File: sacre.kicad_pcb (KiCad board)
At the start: 2 copper layers, 91.4 x 88.4 mm, 72 parts, among them IC1 ST25DV64KC-IE6S3, J1 USB_B_Micro, J2 Conn_01x24, J3 Con_BATT, M1 Vibration_Motor, Q1 DMP1045U_GSD, Q2 UMH3N, Q3 S8050, Q4 SI1308EDL, SW1 SW, SW2 SW, SW3 SW, SW4 SW, U1 TP4054, U2 ADP2108AUJ-3.3, U3 CP2104, U4 LIS3DH, U5 ESP32-PICO-D4, Y1 RV-8803-C7-TA-QC

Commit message: Clean KiCad project files
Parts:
- S1: footprint SamacSys_Parts:MSK12C02 -> MSK12C02:MSK12C02
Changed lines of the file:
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@@
     (pad "3" smd rect locked (at -2.625 -0.85) (size 1 1.55) (layers "F.Cu" "F.Paste" "F.Mask"))
     (pad "4" smd rect locked (at -2.625 0.85) (size 1 1.55) (layers "F.Cu" "F.Paste" "F.Mask"))
-    (model "EVQ-PUA02K.stp"
-      (offset (xyz 0 0 0))
-      (scale (xyz 1 1 1))
-      (rotate (xyz 0 0 0))
-    )
-    (model "${KICAD6_3DMODEL_DIR}/EVQ-PUA02K.3dshapes/EVQ-PUA02K.stp"
+    (model "${KIPRJMOD}/EVQ-PUA02K/EVQ-PUA02K.stp"
       (offset (xyz 0 0 0))
       (scale (xyz 1 1 1))
@@
     (pad "3" smd rect locked (at -2.625 -0.85 180) (size 1 1.55) (layers "F.Cu" "F.Paste" "F.Mask"))
     (pad "4" smd rect locked (at -2.625 0.85 180) (size 1 1.55) (layers "F.Cu" "F.Paste" "F.Mask"))
-    (model "EVQ-PUA02K.stp"
-      (offset (xyz 0 0 0))
-      (scale (xyz 1 1 1))
-      (rotate (xyz 0 0 0))
-    )
-    (model "${KICAD6_3DMODEL_DIR}/EVQ-PUA02K.3dshapes/EVQ-PUA02K.stp"
+    (model "${KIPRJMOD}/EVQ-PUA02K/EVQ-PUA02K.stp"
       (offset (xyz 0 0 0))
       (scale (xyz 1 1 1))
@@
     (pad "3" smd rect locked (at -2.625 -0.85 180) (size 1 1.55) (layers "F.Cu" "F.Paste" "F.Mask"))
     (pad "4" smd rect locked (at -2.625 0.85 180) (size 1 1.55) (layers "F.Cu" "F.Paste" "F.Mask"))
-    (model "EVQ-PUA02K.stp"
-      (offset (xyz 0 0 0))
-      (scale (xyz 1 1 1))
-      (rotate (xyz 0 0 0))
-    )
-    (model "${KICAD6_3DMODEL_DIR}/EVQ-PUA02K.3dshapes/EVQ-PUA02K.stp"
+    (model "${KIPRJMOD}/EVQ-PUA02K/EVQ-PUA02K.stp"
       (offset (xyz 0 0 0))
       (scale (xyz 1 1 1))
@@
     (pad "2" smd rect locked (at 1.425 0 90) (size 1.55 3) (layers "F.Cu" "F.Paste" "F.Mask")
       (net 4 "+3V3") (pintype "passive"))
-    (model "LQH44PN100MP0L.stp"
-      (offset (xyz 0 0 0))
-      (scale (xyz 1 1 1))
-      (rotate (xyz 0 0 0))
-    )
   )
   (footprint "Diode_SMD:D_SOD-123" locked (layer "F.Cu")
@@
     )
   )
-  (footprint "SamacSys_Parts:MSK12C02" locked (layer "F.Cu")
+  (footprint "MSK12C02:MSK12C02" locked (layer "F.Cu")
     (at 53.7 156.5)
     (descr "MSK12C02-1")
@@
     (pad "MP4" smd rect locked (at -3.45 -1.05 90) (size 0.5 0.8) (layers "F.Cu" "F.Paste" "F.Mask")
       (net 56 "Net-(S1-PadMP1)") (pinfunction "MP4") (pintype "passive"))
-    (model "C:\\Users\\Cosmin\\Desktop\\KiCadLib\\SamacSys_Parts.3dshapes\\MSK12C02.stp"
-      (offset (xyz 0 0 0.7))
-      (scale (xyz 1 1 1))
-      (rotate (xyz -90 0 0))
-    )
   )
   (footprint "Inductor_SMD:L_0805_2012Metric_Pad1.15x1.40mm_HandSolder" locked (layer "F.Cu")
@@
     (pad "3" smd rect locked (at -2.625 -0.85) (size 1 1.55) (layers "F.Cu" "F.Paste" "F.Mask"))
     (pad "4" smd rect locked (at -2.625 0.85) (size 1 1.55) (layers "F.Cu" "F.Paste" "F.Mask"))
-    (model "EVQ-PUA02K.stp"
-      (offset (xyz 0 0 0))
-      (scale (xyz 1 1 1))
-      (rotate (xyz 0 0 0))
-    )
-    (model "${KICAD6_3DMODEL_DIR}/EVQ-PUA02K.3dshapes/EVQ-PUA02K.stp"
-      (offset (xyz 0 0 0))
-      (scale (xyz 1 1 1))
+    (model "${KIPRJMOD}/EVQ-PUA02K/EVQ-PUA02K.stp"
+      (offset (xyz 0 0 0))
+      (scale (xyz 1 1 1))

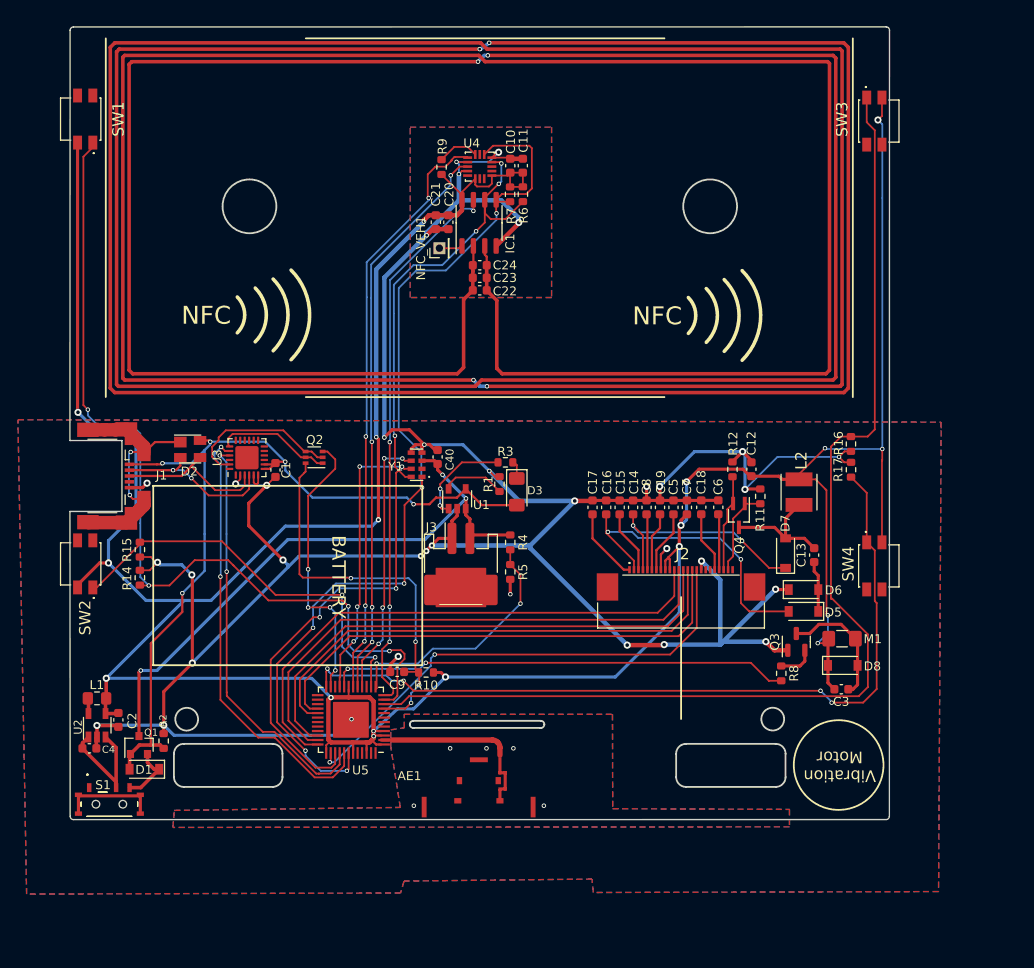
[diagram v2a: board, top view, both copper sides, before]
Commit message: se fini
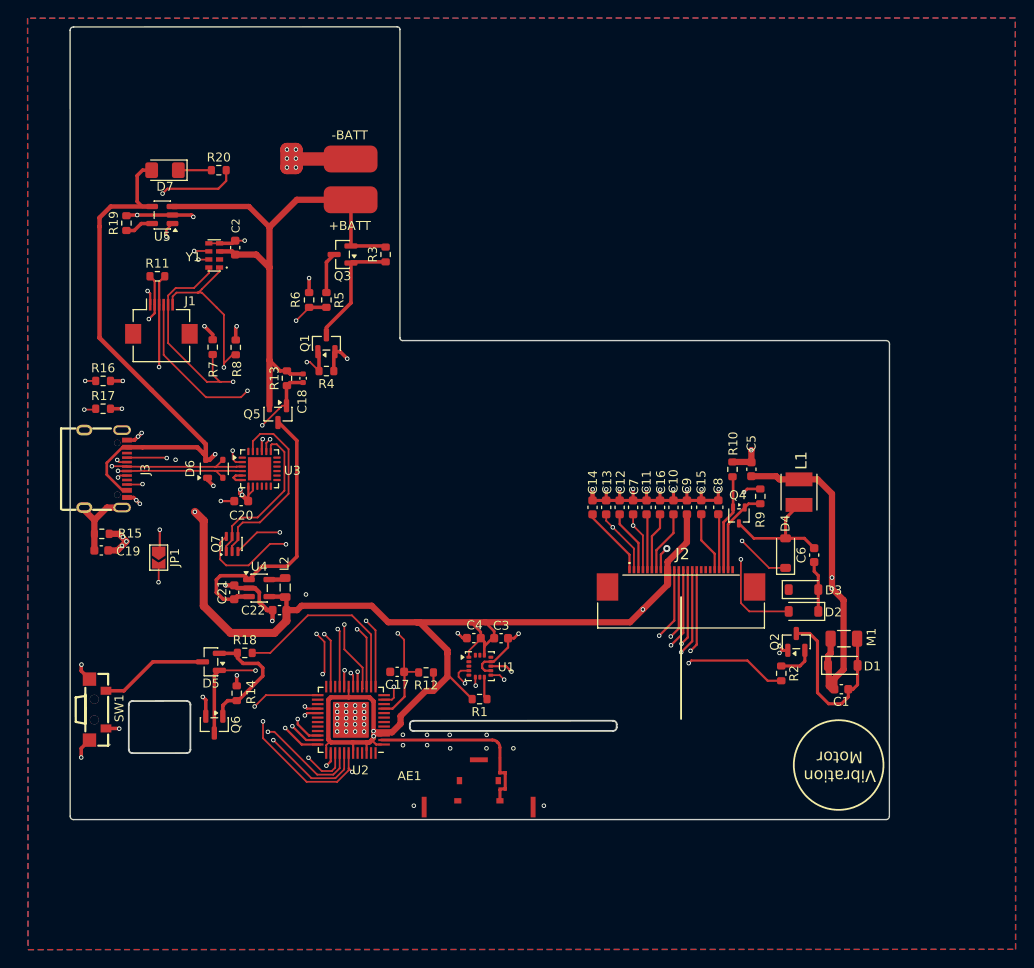
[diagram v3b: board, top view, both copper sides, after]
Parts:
- removed the C1 at (72.2, 119.2)
- removed the C10 at (98.4, 85.3)
- removed the C11 at (99.8, 85.3)
- removed the C2 at (54.7, 147.1)
- removed C23, C24: C_Tune, Capacitor_SMD:C_0603_1608Metric
- removed the D1 at (57.6, 152.6)
- removed the D2 at (62.7, 116.9)
- removed the D3 at (99.1, 121.7)
- removed IC1: ST25DV64KC-IE6S3, Package_SO:SO-8_3.9x4.9mm_P1.27mm
- removed the L1 at (52.3, 144.7)
- removed NFC_VEH1: Conn_01x01_Female, Connector_PinHeader_2.00mm:PinHeader_1x01_P2.00mm_Vertical
- removed the Q2 at (76.5, 117.8)
- removed the R2 at (59.8, 149.4)
- removed the R9 at (90.7, 85.5)
- removed S1: MSK12C02, MSK12C02:MSK12C02
- removed SW2, SW3, SW4: SW, EVQ-PUA02K:EVQPUA02K
- removed the U2 at (52.3, 147.7)
- added C18: 100nF, Capacitor_SMD:C_0402_1005Metric, F.Cu at (75.3, 109.0)
- added C19: 4.7nF, Capacitor_SMD:C_0603_1608Metric, F.Cu at (52.8, 128.2)
- added C3: 0.1uF, Capacitor_SMD:C_0603_1608Metric, F.Cu at (97.4, 138.0)
- added D5: BAT54C, Package_TO_SOT_SMD:SOT-23, F.Cu at (65.0, 140.6)
- added D6: SP0503BAHTG, Package_TO_SOT_SMD:SOT-143, F.Cu at (65.4, 119.1)
- added D7: LED, LED_SMD:LED_1206_3216Metric_Pad1.42x1.75mm_HandSolder, F.Cu at (59.9, 85.8)
- added J5: +BATT, Connector_Wire:SolderWirePad_1x01_SMD_3x6mm, F.Cu at (80.6, 89.1)
- added J6: -BATT, Connector_Wire:SolderWirePad_1x01_SMD_3x6mm, F.Cu at (80.6, 84.5)
- added JP1: Jumper_RES_Touch, Jumper:SolderJumper-2_P1.3mm_Open_TrianglePad1.0x1.5mm, F.Cu at (59.2, 129.0)
- added L2: 1uH, Inductor_SMD:L_0805_2012Metric, F.Cu at (73.3, 132.3)
- added Q3: CJ3415, Package_TO_SOT_SMD:SOT-23, F.Cu at (79.7, 95.2)
- added Q5: CJ3415, Package_TO_SOT_SMD:SOT-23, F.Cu at (72.5, 113.0)
- added Q6: CJ2312, Package_TO_SOT_SMD:SOT-23, F.Cu at (65.4, 147.6)
- added Q7: UMH3N, Package_TO_SOT_SMD:SOT-363_SC-70-6, F.Cu at (67.4, 127.5)
- added R11: 10K, Resistor_SMD:R_0603_1608Metric, F.Cu at (59.0, 97.6)
- added R13: 300k, Resistor_SMD:R_0603_1608Metric, F.Cu at (73.5, 109.0)
- added R18: 1k, Resistor_SMD:R_0603_1608Metric, F.Cu at (68.8, 139.6)
- added R19: 10K, Resistor_SMD:R_0603_1608Metric, F.Cu at (55.6, 91.7)
- added R20: 1K, Resistor_SMD:R_0603_1608Metric, F.Cu at (65.9, 85.8)
- added R6: 10K, Resistor_SMD:R_0603_1608Metric, F.Cu at (76.0, 100.3)
- added U5: TP4054, Package_TO_SOT_SMD:SOT-23-5, F.Cu at (59.6, 90.8)
- C20: value 10uF -> 1uF
- C21: value 0.1uF -> 10uF
- C22: value C_Tune -> 10uF
- J1: value USB_B_Micro -> Touch; footprint Custom_USB:USB_Micro_CustomV2 -> Connector_FFC-FPC:Hirose_FH12-6S-0.5SH_1x06-1MP_P0.50mm_Horizontal
- J2: value Conn_01x24 -> Screen
- J3: value Con_BATT -> USB_C_Receptacle_USB2.0_16P; footprint Connector_JST_Custom:JST_PH_S2B-PH-SM4-TB_1x02-1MP_P2.00mm_Horizontal -> EasyEDA:USB-C-SMD_TYPE-C-16PIN-2MD-073
- M1: footprint Capacitor_SMD:C_1206_3216Metric_Pad1.42x1.75mm_HandSolder -> Capacitor_SMD:C_1206_3216Metric
- Q1: value DMP1045U_GSD -> CJ2312
- Q4: footprint Package_TO_SOT_SMD:SOT-323_SC-70_Handsoldering -> Package_TO_SOT_SMD:SOT-323_SC-70
- R14: value 10K -> 100K
- R15: value 10K -> 1M0
- R16, R17: value 10K -> 5.1k
- R3: value 1K -> 100K
- R5: value 100K -> 10K
- SW1: value SW -> TSC02-TDW1FH3.5; footprint EVQ-PUA02K:EVQPUA02K -> EasyEDA:SW-SMD_L7.8-W3.5-P4.20-EH
- U1: value TP4054 -> LIS3DH; footprint Package_TO_SOT_SMD:SOT-23-5 -> Package_LGA:LGA-16_3x3mm_P0.5mm_LayoutBorder3x5y
- U4: value LIS3DH -> ADP2108AUJ-3.3; footprint LIS3DH:LGA-16_3x3mm_P0.5mm_LayoutBorder3x5y_custom -> Package_TO_SOT_SMD:TSOT-23-5
- moved R16 83.7 mm to (53.0, 109.3), turned to 0 degrees
- moved R17 83.7 mm to (53.0, 112.4), turned to 0 degrees
- moved SW1 65.9 mm to (52.4, 145.9), turned to 90 degrees
- moved U4 53.0 mm to (70.4, 132.4), turned to 0 degrees
- moved Q1 49.4 mm to (77.9, 105.1)
- moved C21 47.0 mm to (67.6, 132.9)
- moved C4 44.6 mm to (94.3, 138.0)
- moved C22 42.1 mm to (72.7, 134.9), turned to 0 degrees
- moved J3 41.0 mm to (53.3, 119.1), turned to -90 degrees
- moved C20 38.7 mm to (68.4, 122.7), turned to 0 degrees
- moved R7 38.6 mm to (65.2, 105.5)
- moved R5 36.6 mm to (77.9, 100.3)
- moved R8 35.0 mm to (67.8, 105.6)
- moved C2 32.5 mm to (67.7, 94.4)
- moved Y1 32.5 mm to (65.4, 95.3)
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- renumbered C3 to C1, C5 to C10, C8 to C11, C15 to C12, C16 to C13, C17 to C14, C18 to C15, C19 to C16, C9 to C17, C40 to C2, C12 to C5, C13 to C6, C14 to C7, C6 to C8, C7 to C9, D8 to D1, D5 to D2, D6 to D3, D7 to D4, L2 to L1, Q3 to Q2, R12 to R10, R10 to R12, R8 to R2, R6 to R7, R7 to R8, R11 to R9, U5 to U2
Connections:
- net Net-(AE1-Pad1) renamed /ANT_RF
- C2 pad 1: +BATT -> VBAT_RAW
- C20 pad 1: +3V3 -> GND
- C20 pad 2: GND -> USB_VBUS
- C21 pad 1: +3V3 -> GND
- C21 pad 2: GND -> VSYS
- C22 pad 1: /NFC_antenna -> GND
- C22 pad 2: /NFC_antenna -> +3V3
- C4 pad 1: GND -> +3V3
- C4 pad 2: Net-(C4-Pad2) -> GND
- J1 pad 1: VBUS -> GND
- J1 pad 2: Net-(D2-Pad2) -> +3V3
- J1 pad 3: Net-(D2-Pad3) -> Net-(J1-Pin_3)
- J1 pad 4: unconnected-(J1-Pad4) -> INT_TOUCH
- J1 pad 5: GND -> SCL
- J1 pad 6: Net-(D2-Pad1) -> SDA
- Q1 pad 1: VBUS -> VBAT_SENSE_EN
- Q1 pad 2: Net-(D1-Pad1) -> GND
- Q1 pad 3: +BATT -> Net-(Q1-D)
- R1 pad 1: Net-(R1-Pad1) -> Net-(U1-CS)
- R1 pad 2: GND -> +3V3
- R14 pad 1: SW_1 -> Net-(Q6-G)
- R15 pad 1: SW_2 -> Net-(J3-SHIELD)
- R16 pad 1: SW_3 -> Net-(J3-CC1)
- R17 pad 1: SW_4 -> Net-(J3-CC2)
- R3 pad 1: Net-(D3-Pad1) -> Net-(Q1-D)
- R3 pad 2: Net-(R3-Pad2) -> VBAT_RAW
- R4 pad 1: +BATT -> GND
- R4 pad 2: ADC_BATT -> VBAT_SENSE_EN
- R5 pad 1: ADC_BATT -> Net-(Q3-D)
- R5 pad 2: GND -> ADC_BATT
- SW1 pad 1: SW_1 -> GND
- SW1 pad 2: +3V3 -> Net-(D5-Pad3)
- U1 pad 1: Net-(R3-Pad2) -> +3V3
- U1 pad 2: GND -> unconnected-(U1-NC-Pad2)
- U1 pad 3: +BATT -> unconnected-(U1-NC-Pad3)
- U1 pad 4: VBUS -> SCL
- U1 pad 5: Net-(R1-Pad1) -> GND
- U2 pad 10: SW_3 -> unconnected-(U2-IO34-Pad10)
- U2 pad 11: SW_1 -> INT_TOUCH
- U2 pad 14: SW_2 -> PWR_BTN
- U2 pad 15: unconnected-(U5-Pad15) -> VBAT_SENSE_EN
- U2 pad 24: SW_4 -> unconnected-(U2-IO4-Pad24)
- U2 pad 25: unconnected-(U5-Pad25) -> RES_TOUCH
- U3 pad 3: Net-(D2-Pad3) -> /Power/USB_D+
- U3 pad 4: Net-(D2-Pad2) -> /Power/USB_D-
- U3 pad 7: VBUS -> USB_VBUS
- U3 pad 8: VBUS -> USB_VBUS
- U4 pad 1: +3V3 -> VSYS
- U4 pad 2: (no net) -> GND
- U4 pad 3: (no net) -> VSYS
- U4 pad 4: SCL -> +3V3
- U4 pad 5: GND -> Net-(U4-SW)
- Y1 pad 3: +BATT -> VBAT_RAW
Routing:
- net /NFC_antenna: track 961.2 -> 0.00 mm, vias 6 -> 0
- net GND: track 347.2 -> 109.7 mm, vias 40 -> 81
- net +3V3: track 389.4 -> 246.6 mm, vias 18 -> 9
- net SW_3: track 126.7 -> 0.00 mm
- net SW_1: track 99.7 -> 0.00 mm, vias 4 -> 0
- net VBUS: track 95.9 -> 0.00 mm, vias 5 -> 0
- net SW_4: track 90.7 -> 0.00 mm, vias 4 -> 0
- net USB_VBUS: track 0.00 -> 74.2 mm, vias 0 -> 3
- net +BATT: track 68.0 -> 0.00 mm, vias 3 -> 0
- net INT_TOUCH: track 0.00 -> 64.1 mm, vias 0 -> 4
- net GPO: track 62.3 -> 0.00 mm, vias 4 -> 0
- net VBAT_RAW: track 0.00 -> 61.8 mm
- net Net-(Q5-G): track 0.00 -> 52.9 mm, vias 0 -> 2
- net VBAT_SENSE_EN: track 0.00 -> 46.5 mm, vias 0 -> 2
- net SW_2: track 46.3 -> 0.00 mm, vias 2 -> 0
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- added copper zone on In1.Cu, net GND
- added copper zone on In2.Cu, net GND
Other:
- outline, holes or cut-outs redrawn
- copper layers 2 -> 4
- board text removed: "BATTERY"
- board text removed: "NFC"
